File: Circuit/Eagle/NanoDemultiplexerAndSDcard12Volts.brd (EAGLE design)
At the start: 100 x 70 mm, 68 parts

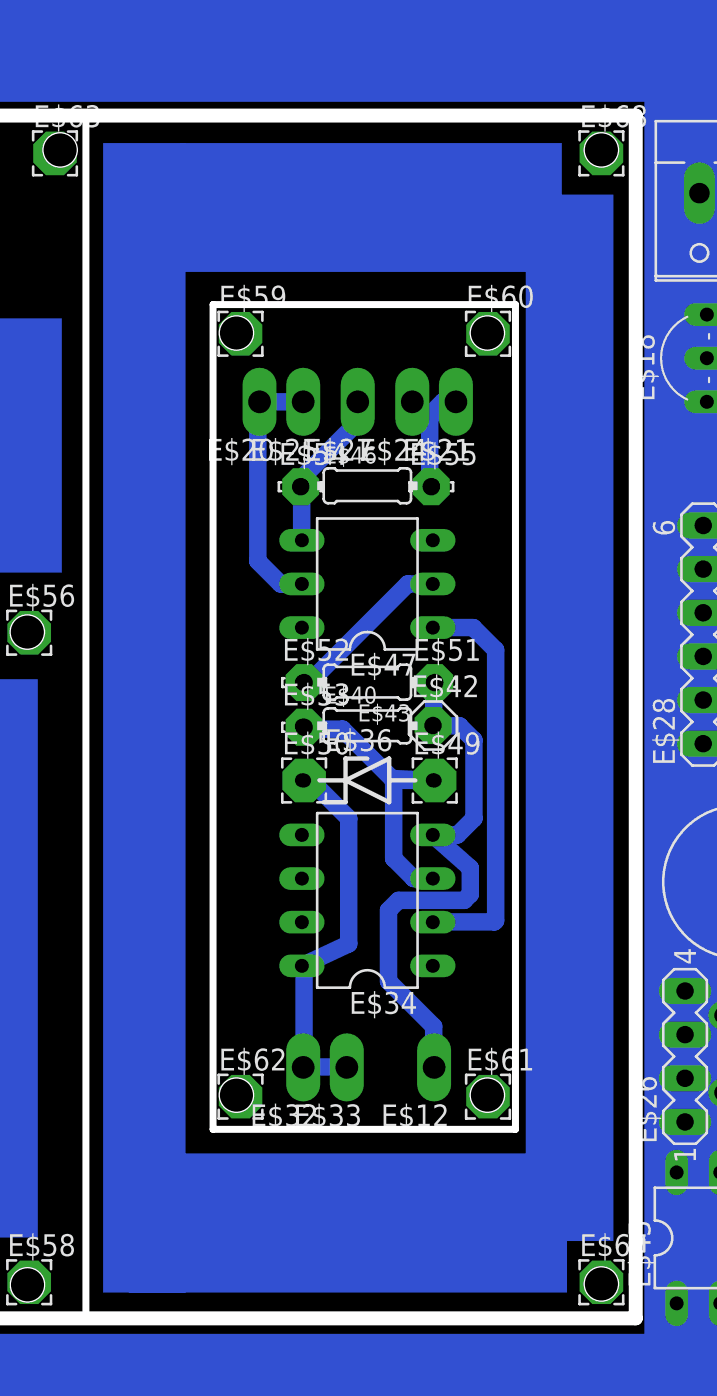
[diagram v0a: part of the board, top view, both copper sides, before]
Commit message: .
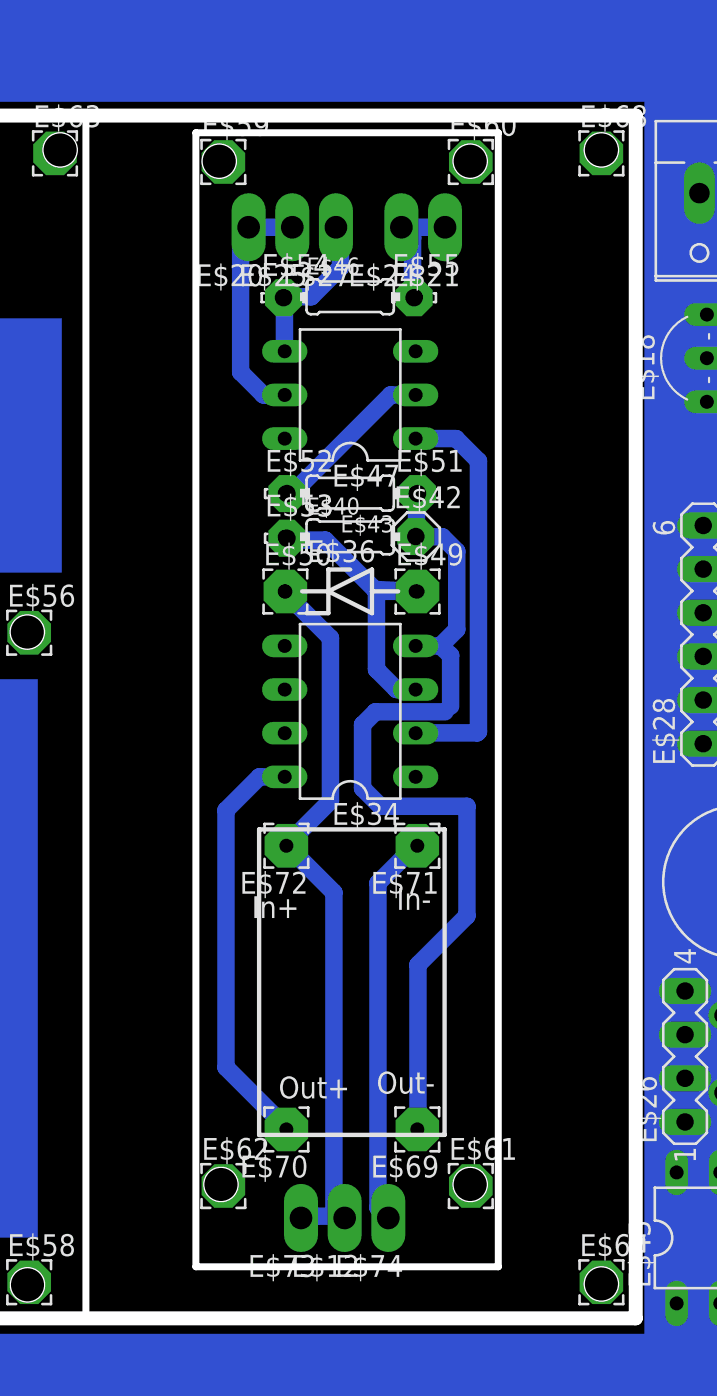
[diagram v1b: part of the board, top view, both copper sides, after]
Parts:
- removed E$32, E$33: (no value), testpad:P1-13Y
- added E$69, E$70, E$71, E$72: (no value), wirepad:2,54/0,8
- added E$73, E$74: (no value), testpad:P1-13Y
- E$40: value 220 -> 1k
- moved E$50 11.1 mm to (79.6, 42.3)
- moved E$34 11.0 mm to (83.4, 35.3)
- moved E$36 11.0 mm to (83.4, 42.3)
- moved E$40 11.0 mm to (83.4, 45.5)
- moved E$42 11.0 mm to (87.2, 45.5)
- moved E$43 11.0 mm to (83.4, 48.0)
- moved E$46 11.0 mm to (83.4, 59.5)
- moved E$47 11.0 mm to (83.4, 53.7)
- moved E$51 11.0 mm to (87.3, 48.0)
- moved E$52 11.0 mm to (79.7, 48.0)
- moved E$53 11.0 mm to (79.7, 45.4)
- moved E$54 11.0 mm to (79.5, 59.4)
- moved E$55 11.0 mm to (87.1, 59.4)
- moved E$49 11.0 mm to (87.3, 42.3)
- moved E$27 10.2 mm to (82.5, 63.5)
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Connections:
- net S$38 renamed S$10
- new net 0V: E$71.1, E$74.TP
- new net 12V: E$12.TP, E$36.C, E$72.1, E$73.TP
- new net S$32: E$21.TP, E$24.TP, E$46.2
- new net S$33: E$20.TP, E$25.TP
- new net S$9: E$47.5
- net 5V: no longer E$20.TP, E$25.TP, E$47.5
- net B+: now also E$70.1; no longer E$32.TP, E$33.TP, E$36.C
- net B-: now also E$69.1; no longer E$12.TP
- net GND: no longer E$21.TP, E$24.TP, E$46.2
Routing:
- net 12V: track 0.00 -> 43.3 mm
- net 0V: track 0.00 -> 22.9 mm
- net B-: track 32.5 -> 52.2 mm
- net 5V: track 126.8 -> 111.8 mm
- net S$9: track 0.00 -> 11.6 mm
- net GND: track 118.5 -> 109.5 mm
- net S$32: track 0.00 -> 7.08 mm
- net S$33: track 0.00 -> 2.54 mm
- net B+: track 22.6 -> 24.2 mm
- net S$44: track 9.74 -> 10.4 mm
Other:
- outline, holes or cut-outs redrawn
- board text added: "In+"
- board text added: "In-"
- board text added: "Out+"
- board text added: "Out-"
- board text removed: "5v"
- board text removed: "mi"
- board text removed: "mo"
- board text removed: "sck"
